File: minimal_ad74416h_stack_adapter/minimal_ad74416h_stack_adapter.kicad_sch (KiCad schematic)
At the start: 6 parts, among them J1 CLP-133-02-G-D-BE, J2 CLP-133-02-G-D-BE, J3 CLP-133-02-G-D-BE, J4 CLP-133-02-G-D-BE, J5 CLP-133-02-G-D-BE, J6 FW-33-03-G-D-085-155

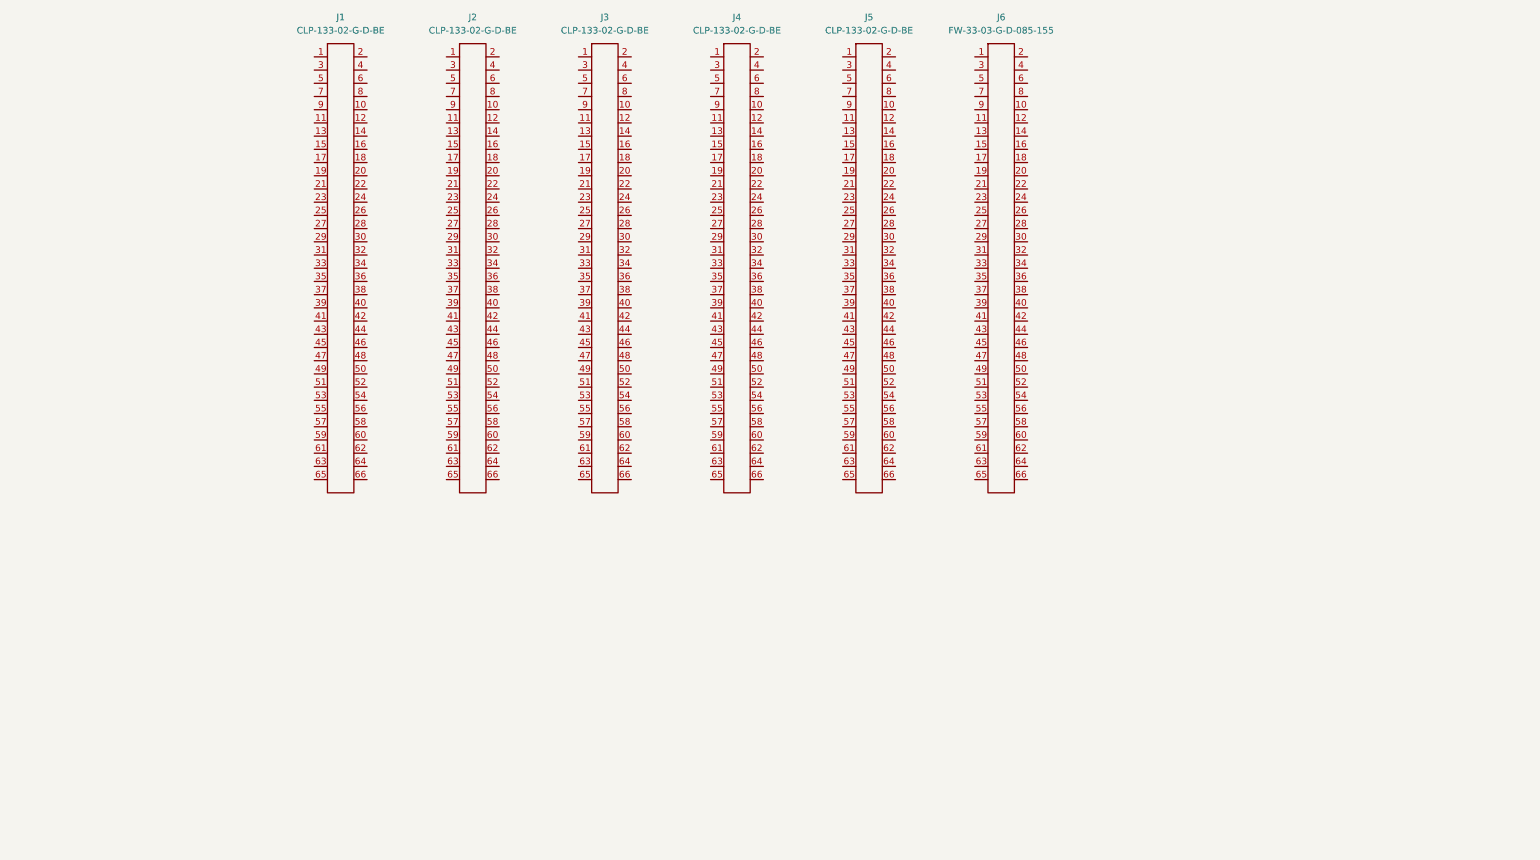
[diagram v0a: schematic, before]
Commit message: backup
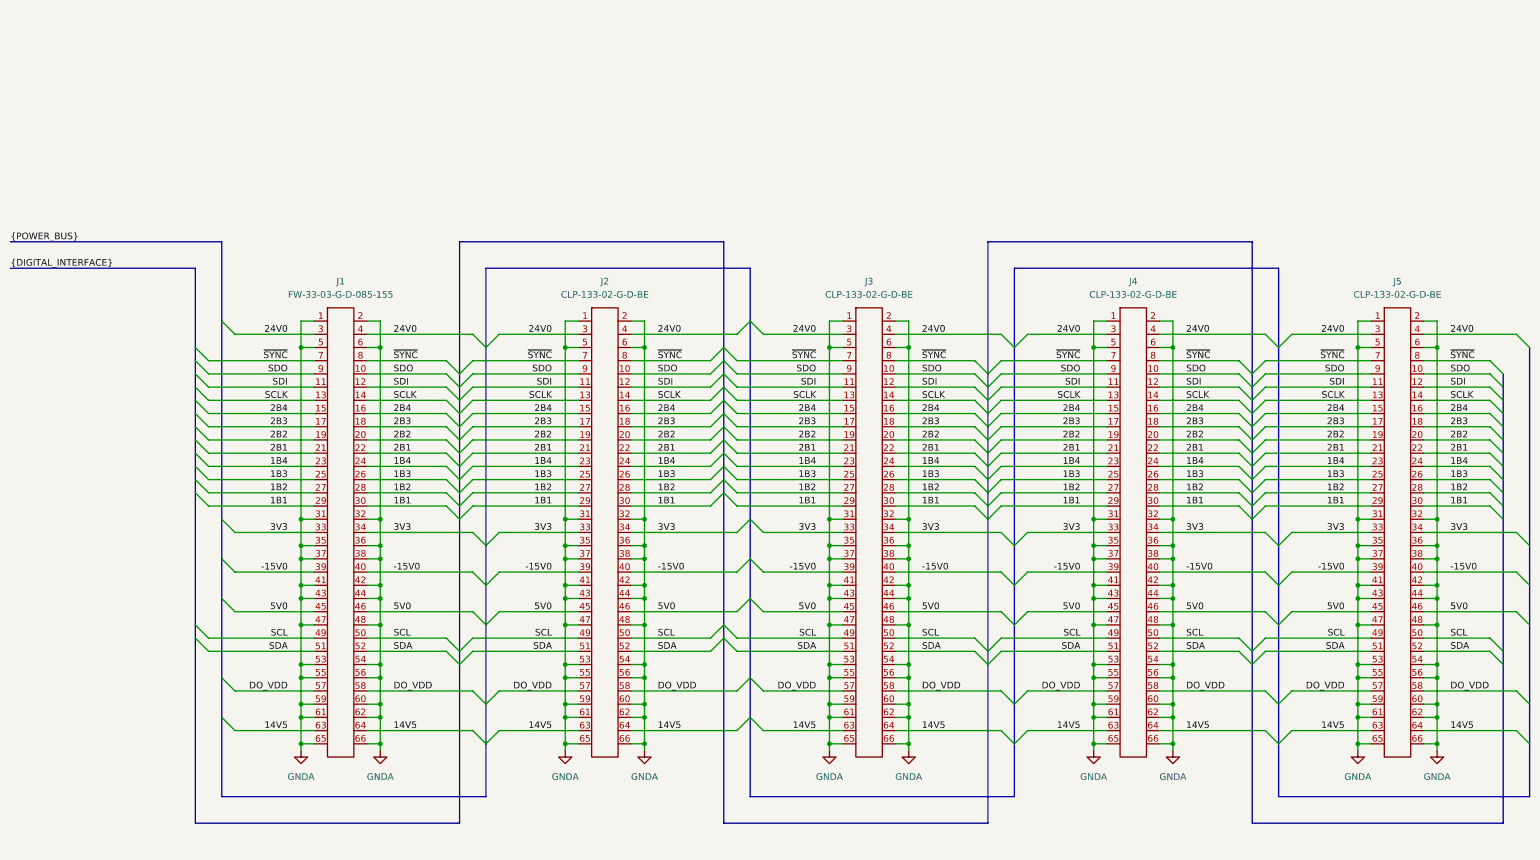
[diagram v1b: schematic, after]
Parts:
- removed J4: CLP-133-02-G-D-BE, connector_footprints:CLP-133-02-G-D-BE, symbol CONNECTORS_CLP-1xx-02-G-D-BE_DATA_BASE:J_CLP-133-02-G-D-BE
- J1: value CLP-133-02-G-D-BE -> FW-33-03-G-D-085-155; footprint connector_footprints:CLP-133-02-G-D-BE -> connector_footprints:FW-33-03-G-D-085-155; Contact Plating Tin -> Gold; MPN CLP-133-02-G-D-BE -> FW-33-03-G-D-085-155; Series CLP-1xx-02-G-D-BE -> FW-xx-03-G-D-085-155; Symbol Name J_CLP-133-02-G-D-BE -> J_FW-33-03-G-D-085-155; Trustedparts Search https://www.trustedparts.com/en/search/CLP-133-02-G-D-BE -> https://www.trustedparts.com/en/search/FW-33-03-G-D-085-155
- J4: renamed from J6; value FW-33-03-G-D-085-155 -> CLP-133-02-G-D-BE; footprint connector_footprints:FW-33-03-G-D-085-155 -> connector_footprints:CLP-133-02-G-D-BE; Color Black -> (none); Contact Plating Gold -> (none); Current Rating (A) 5.2 -> (none); MPN FW-33-03-G-D-085-155 -> (none); Manufacturer Samtec -> (none); Mounting Angle Vertical -> (none); Mounting Style Surface Mount -> (none); Number of Rows 2 -> (none); Pin Count 33 -> (none); Pitch (mm) 1.27 -> (none); Series FW-xx-03-G-D-085-155 -> (none); Symbol Name J_FW-33-03-G-D-085-155 -> (none); Trustedparts Search https://www.trustedparts.com/en/search/FW-33-03-G-D-085-155 -> (none); Voltage Rating (V) 300 -> (none)
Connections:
- net GNDA: now reaches J3.1
- net GNDA: now also J1.1, J1.2, J1.31, J1.32, J1.35, J1.36, J1.37, J1.38, J1.41, J1.42, J1.43, J1.44, J1.47, J1.48, J1.5, J1.53, J1.54, J1.55, J1.56, J1.59, J1.6, J1.60, J1.61, J1.62, J1.65, J1.66, J2.1, J2.2, J2.31, J2.32, J2.35, J2.36, J2.37, J2.38, J2.41, J2.42, J2.43, J2.44, J2.47, J2.48, J2.5, J2.53, J2.54, J2.55, J2.56, J2.59, J2.6, J2.60, J2.61, J2.62, J2.65, J2.66, J3.2, J3.31, J3.32, J3.35, J3.36, J3.37, J3.38, J3.41, J3.42, J3.43, J3.44, J3.47, J3.48, J3.5, J3.53, J3.54, J3.55, J3.56, J3.59, J3.6, J3.60, J3.61, J3.62, J3.65, J3.66, J4.1, J4.2, J4.31, J4.32, J4.35, J4.36, J4.37, J4.38, J4.41, J4.42, J4.43, J4.44, J4.47, J4.48, J4.5, J4.53, J4.54, J4.55, J4.56, J4.59, J4.6, J4.60, J4.61, J4.62, J4.65, J4.66, J5.1, J5.2, J5.31, J5.32, J5.35, J5.36, J5.37, J5.38, J5.41, J5.42, J5.43, J5.44, J5.47, J5.48, J5.5, J5.53, J5.54, J5.55, J5.56, J5.59, J5.6, J5.60, J5.61, J5.62, J5.65, J5.66
- net SDO: now reaches J3.10
- net SDO: now also J1.10, J1.9, J2.10, J2.9, J3.9, J4.10, J4.9, J5.10, J5.9
- net SDI: now reaches J3.11
- net SDI: now also J1.11, J1.12, J2.11, J2.12, J3.12, J4.11, J4.12, J5.11, J5.12
- net SCLK: now reaches J3.13
- net SCLK: now also J1.13, J1.14, J2.13, J2.14, J3.14, J4.13, J4.14, J5.13, J5.14
- net 2B4: now reaches J3.15
- net 2B4: now also J1.15, J1.16, J2.15, J2.16, J3.16, J4.15, J4.16, J5.15, J5.16
- net 2B3: now reaches J3.17
- net 2B3: now also J1.17, J1.18, J2.17, J2.18, J3.18, J4.17, J4.18, J5.17, J5.18
- net 2B2: now reaches J3.19
- net 2B2: now also J1.19, J1.20, J2.19, J2.20, J3.20, J4.19, J4.20, J5.19, J5.20
- net 2B1: now reaches J3.21
- net 2B1: now also J1.21, J1.22, J2.21, J2.22, J3.22, J4.21, J4.22, J5.21, J5.22
- net 1B4: now reaches J3.23
- net 1B4: now also J1.23, J1.24, J2.23, J2.24, J3.24, J4.23, J4.24, J5.23, J5.24
- net 1B3: now reaches J3.25
- net 1B3: now also J1.25, J1.26, J2.25, J2.26, J3.26, J4.25, J4.26, J5.25, J5.26
- net 1B2: now reaches J3.27
- net 1B2: now also J1.27, J1.28, J2.27, J2.28, J3.28, J4.27, J4.28, J5.27, J5.28
- net 1B1: now reaches J3.29
- net 1B1: now also J1.29, J1.30, J2.29, J2.30, J3.30, J4.29, J4.30, J5.29, J5.30
- net 24V0: now reaches J3.3
- net 24V0: now also J1.3, J1.4, J2.3, J2.4, J3.4, J4.3, J4.4, J5.3, J5.4
- net 3V3: now reaches J3.33
- net 3V3: now also J1.33, J1.34, J2.33, J2.34, J3.34, J4.33, J4.34, J5.33, J5.34
- net -15V0: now reaches J3.39
- net -15V0: now also J1.39, J1.40, J2.39, J2.40, J3.40, J4.39, J4.40, J5.39, J5.40
- net 5V0: now reaches J3.45
- net 5V0: now also J1.45, J1.46, J2.45, J2.46, J3.46, J4.45, J4.46, J5.45, J5.46
- net SCL: now reaches J3.49
- net SCL: now also J1.49, J1.50, J2.49, J2.50, J3.50, J4.49, J4.50, J5.49, J5.50
- net SDA: now reaches J3.51
- net SDA: now also J1.51, J1.52, J2.51, J2.52, J3.52, J4.51, J4.52, J5.51, J5.52
- net DO_VDD: now reaches J3.57
- net DO_VDD: now also J1.57, J1.58, J2.57, J2.58, J3.58, J4.57, J4.58, J5.57, J5.58
- net 14V5: now reaches J3.63
- net 14V5: now also J1.63, J1.64, J2.63, J2.64, J3.64, J4.63, J4.64, J5.63, J5.64
- net ~{SYNC}: now reaches J3.7
- net ~{SYNC}: now also J1.7, J1.8, J2.7, J2.8, J3.8, J4.7, J4.8, J5.7, J5.8
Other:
- moved on the sheet: J1, J2, J3, J4, J5

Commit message: backup
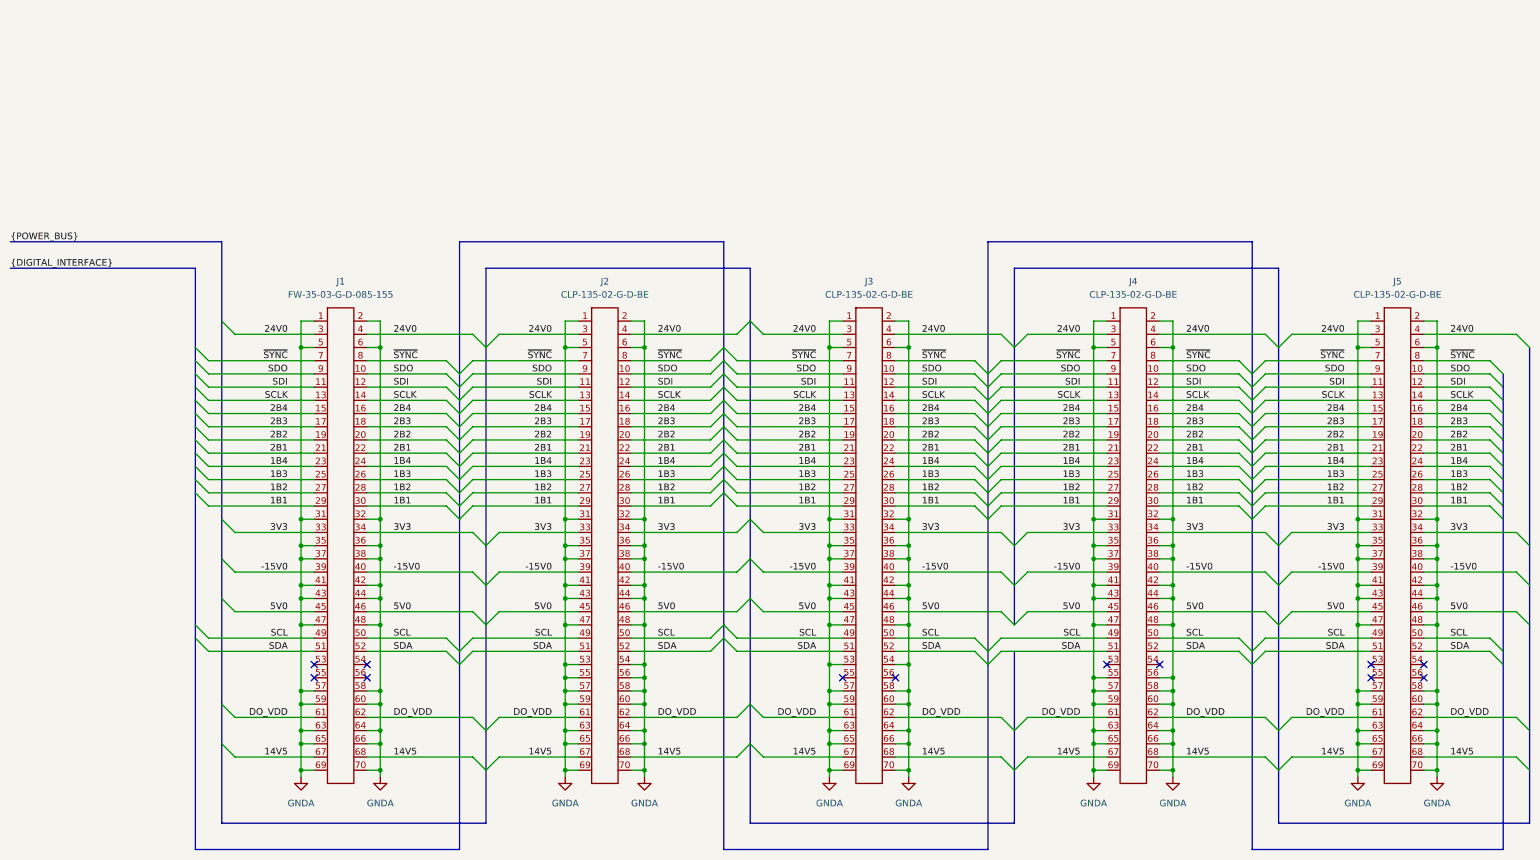
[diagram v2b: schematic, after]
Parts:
- J1: renamed from J4; value CLP-133-02-G-D-BE -> FW-35-03-G-D-085-155; footprint connector_footprints:CLP-133-02-G-D-BE -> connector_footprints:FW-35-03-G-D-085-155; symbol CONNECTORS_FW-xx-03-G-D-085-155_DATA_BASE:J_FW-33-03-G-D-085-155 -> CONNECTORS_FW-xx-03-G-D-085-155_DATA_BASE:J_FW-35-03-G-D-085-155; Color (none) -> Black; Contact Plating (none) -> Gold; Current Rating (A) (none) -> 5.2; MPN (none) -> FW-35-03-G-D-085-155; Manufacturer (none) -> Samtec; Mounting Angle (none) -> Vertical; Mounting Style (none) -> Surface Mount; Number of Rows (none) -> 2; Pin Count (none) -> 35; Pitch (mm) (none) -> 1.27; Series (none) -> FW-xx-03-G-D-085-155; Symbol Name (none) -> J_FW-35-03-G-D-085-155; Trustedparts Search (none) -> https://www.trustedparts.com/en/search/FW-35-03-G-D-085-155; Voltage Rating (V) (none) -> 300
- J2, J3, J5: value CLP-133-02-G-D-BE -> CLP-135-02-G-D-BE; footprint connector_footprints:CLP-133-02-G-D-BE -> connector_footprints:CLP-135-02-G-D-BE; symbol CONNECTORS_CLP-1xx-02-G-D-BE_DATA_BASE:J_CLP-133-02-G-D-BE -> CONNECTORS_CLP-1xx-02-G-D-BE_DATA_BASE:J_CLP-135-02-G-D-BE; MPN CLP-133-02-G-D-BE -> CLP-135-02-G-D-BE; Pin Count 33 -> 35; Symbol Name J_CLP-133-02-G-D-BE -> J_CLP-135-02-G-D-BE; Trustedparts Search https://www.trustedparts.com/en/search/CLP-133-02-G-D-BE -> https://www.trustedparts.com/en/search/CLP-135-02-G-D-BE
- J4: renamed from J1; value FW-33-03-G-D-085-155 -> CLP-135-02-G-D-BE; footprint connector_footprints:FW-33-03-G-D-085-155 -> connector_footprints:CLP-135-02-G-D-BE; symbol CONNECTORS_CLP-1xx-02-G-D-BE_DATA_BASE:J_CLP-133-02-G-D-BE -> CONNECTORS_CLP-1xx-02-G-D-BE_DATA_BASE:J_CLP-135-02-G-D-BE; Contact Plating Gold -> Tin; MPN FW-33-03-G-D-085-155 -> CLP-135-02-G-D-BE; Pin Count 33 -> 35; Series FW-xx-03-G-D-085-155 -> CLP-1xx-02-G-D-BE; Symbol Name J_FW-33-03-G-D-085-155 -> J_CLP-135-02-G-D-BE; Trustedparts Search https://www.trustedparts.com/en/search/FW-33-03-G-D-085-155 -> https://www.trustedparts.com/en/search/CLP-135-02-G-D-BE
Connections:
- net 14V5: now also J1.67, J1.68, J2.67, J2.68, J3.67, J3.68, J4.67, J4.68, J5.67, J5.68; no longer J1.63, J1.64, J2.63, J2.64, J3.63, J3.64, J4.63, J4.64, J5.63, J5.64
- net DO_VDD: now also J1.61, J1.62, J2.61, J2.62, J3.61, J3.62, J4.61, J4.62, J5.61, J5.62; no longer J1.57, J1.58, J2.57, J2.58, J3.57, J3.58, J4.57, J4.58, J5.57, J5.58
- net GNDA: now also J1.57, J1.58, J1.63, J1.64, J1.69, J1.70, J2.57, J2.58, J2.63, J2.64, J2.69, J2.70, J3.57, J3.58, J3.63, J3.64, J3.69, J3.70, J4.57, J4.58, J4.63, J4.64, J4.69, J4.70, J5.57, J5.58, J5.63, J5.64, J5.69, J5.70; no longer J1.53, J1.54, J1.55, J1.56, J1.61, J1.62, J2.61, J2.62, J3.55, J3.56, J3.61, J3.62, J4.53, J4.54, J4.61, J4.62, J5.53, J5.54, J5.55, J5.56, J5.61, J5.62
- no-connect marks 0 -> 12
